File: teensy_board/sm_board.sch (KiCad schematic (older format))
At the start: 45 parts, among them J0 CONN_01X03, J1 CONN_01X03, J10 CONN_01X04, J11 CONN_01X02, J12 CONN_02X04, J2 CONN_01X03, J3 CONN_01X03, J4 CONN_01X03, J5 CONN_01X03, J6 CONN_01X03, J7 CONN_01X02, J8 CONN_01X02, J9 CONN_01X04, U1 Teensy3.6, U2 drv8833, U3 tps82130

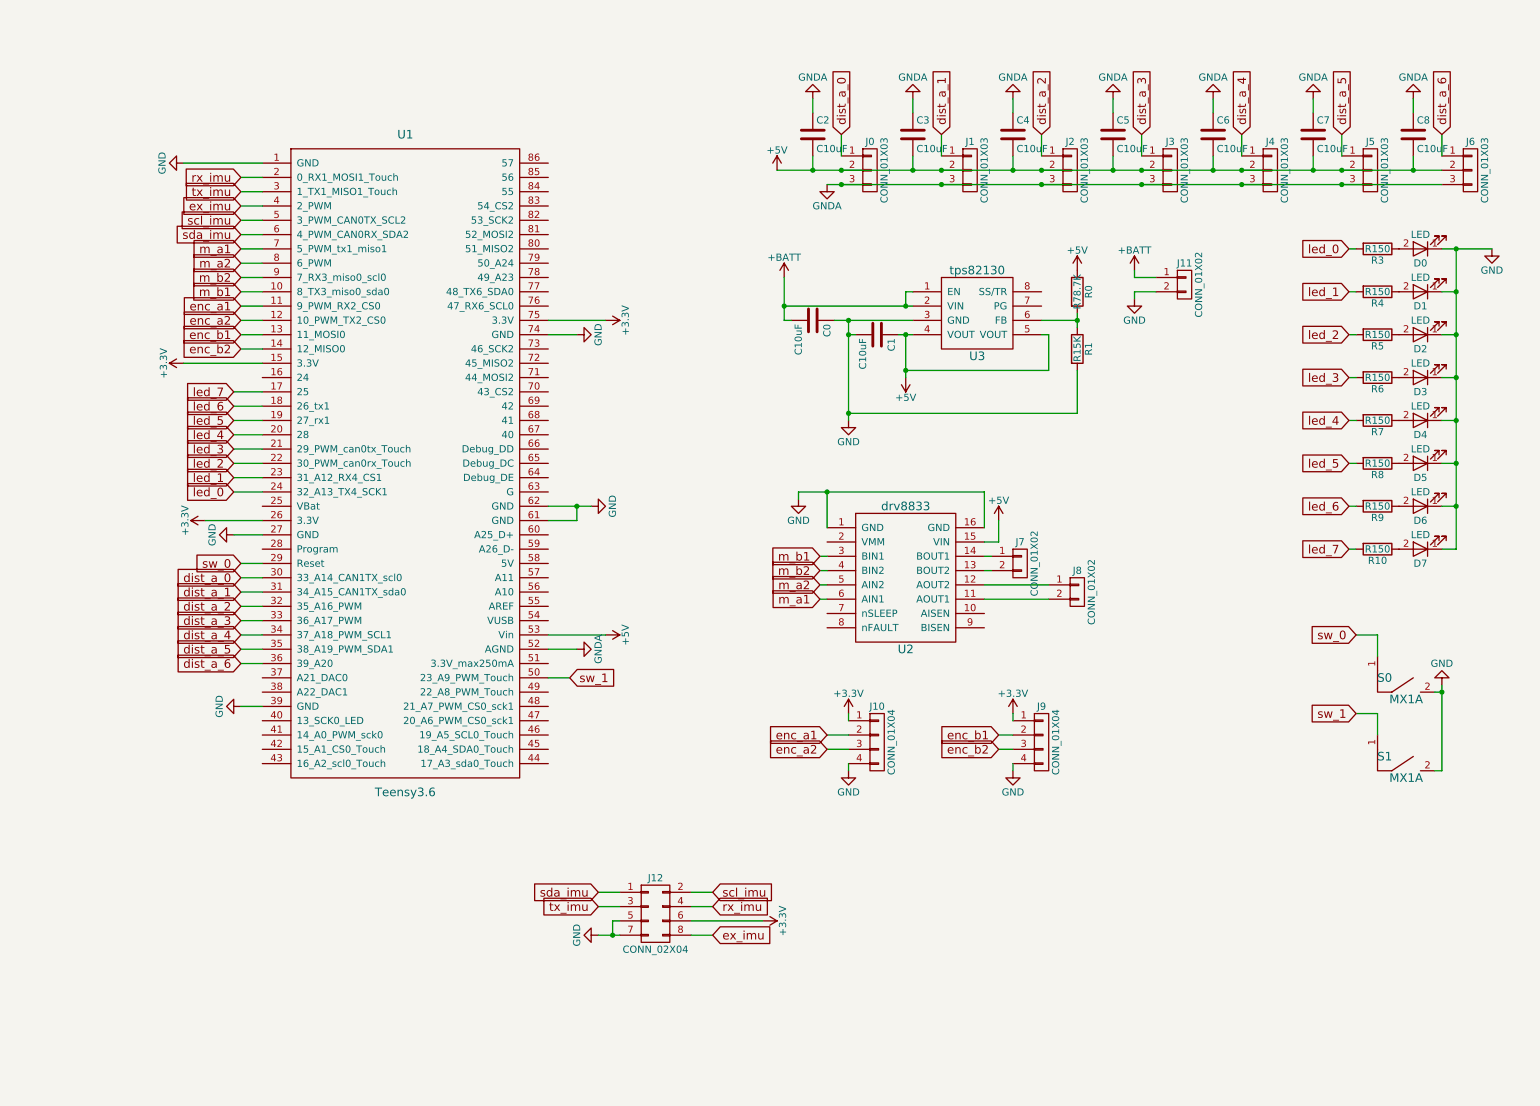
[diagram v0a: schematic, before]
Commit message: I think im done the schematic for tonight
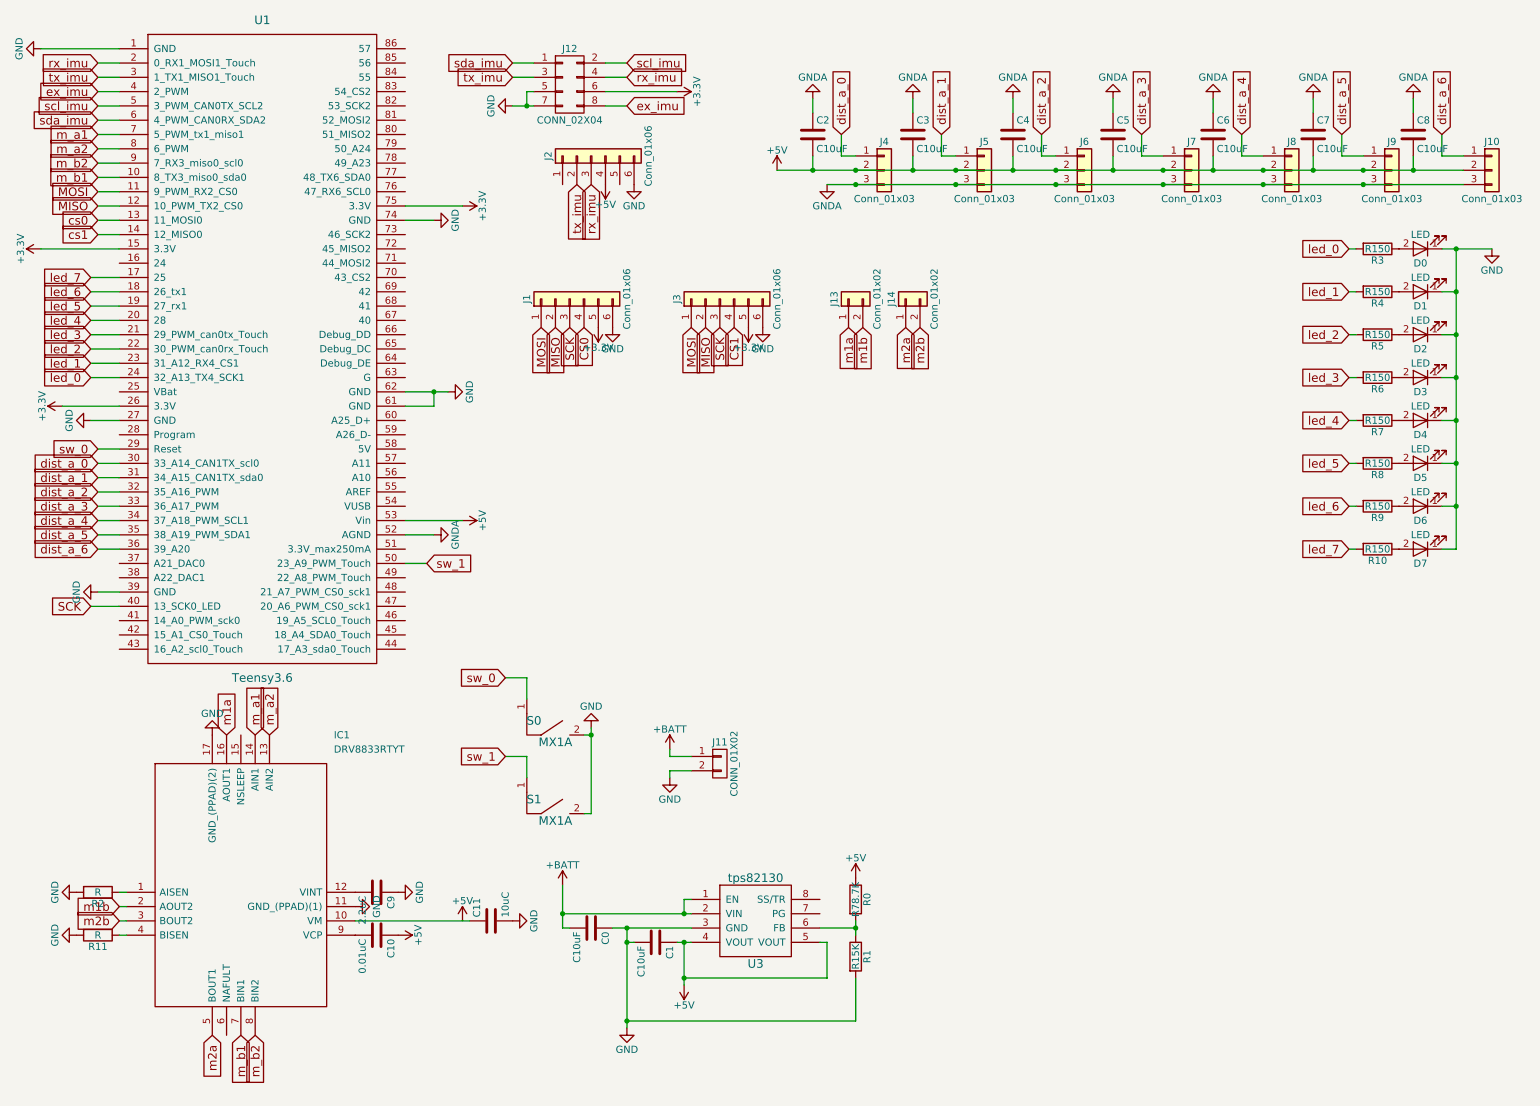
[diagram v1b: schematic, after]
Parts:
- removed J0, J1, J2, J3, J4, J5, J6: CONN_01X03, Pin_Headers:Pin_Header_Straight_1x03_Pitch2.54mm, symbol CONN_01X03
- removed J10, J9: CONN_01X04, Pin_Headers:Pin_Header_Straight_1x04_Pitch2.54mm, symbol CONN_01X04
- removed J7, J8: CONN_01X02, Pin_Headers:Pin_Header_Straight_1x02_Pitch2.54mm, symbol CONN_01X02
- removed U2: drv8833, drv8833:drv8833, symbol drv8833
- added C10: 0.01uC, Capacitors_SMD:C_0603, symbol C
- added C11: 10uC, Capacitors_SMD:C_0603, symbol C
- added C9: 2.2uC, Capacitors_SMD:C_0603, symbol C
- added IC1: DRV8833RTYT, Housings_DFN_QFN:WQFN-16-1EP_4x4mm_Pitch0.65mm, symbol DRV8833RTYT
- added J1, J3: Conn_01x06, Connector_Molex:Molex_CLIK-Mate_502386-0670_1x06_P1.25mm_Horizontal, symbol Conn_01x06
- added J10, J4, J5, J6, J7, J8, J9: Conn_01x03, Connector_Molex:Molex_CLIK-Mate_502386-0370_1x03_P1.25mm_Horizontal, symbol Conn_01x03
- added J13, J14: Conn_01x02, Connector_Molex:Molex_CLIK-Mate_502494-0270_1x02_P2.00mm_Horizontal, symbol Conn_01x02
- added J2: Conn_01x06, Pin_Headers:Pin_Header_Straight_1x06_Pitch2.54mm, symbol Conn_01x06
- added R11, R2: R, Resistors_SMD:R_0603, symbol R
- C0, C1, C2, C3, C4, C5, C6, C7, C8: footprint Capacitors_SMD:C_0805 -> Capacitors_SMD:C_0603
- D0, D1, D2, D3, D4, D5, D6, D7: footprint LEDs:LED_0805 -> LEDs:LED_0603
- R0, R1, R10, R3, R4, R5, R6, R7, R8, R9: footprint Resistors_SMD:R_0805 -> Resistors_SMD:R_0603
- U1: footprint Teensy:Teensy35_36_custom -> Teensy:Teensy35_36
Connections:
- net +3V3: now also J1.5 (Pin_5), J3.5 (Pin_5)
- net +5V: now also C10.1, J10.2 (Pin_2), J2.4 (Pin_4), J4.2 (Pin_2), J5.2 (Pin_2), J6.2 (Pin_2), J7.2 (Pin_2), J8.2 (Pin_2), J9.2 (Pin_2)
- net GND: now also C11.2, C9.1, IC1.11 (GND_(PPAD)(1)), IC1.17 (GND_(PPAD)(2)), J1.6 (Pin_6), J2.6 (Pin_6), J3.6 (Pin_6), R11.2, R2.2
- net GNDA: now also J10.3 (Pin_3), J4.3 (Pin_3), J5.3 (Pin_3), J6.3 (Pin_3), J7.3 (Pin_3), J8.3 (Pin_3), J9.3 (Pin_3)
- net dist_a_0: now also J4.1 (Pin_1)
- net dist_a_1: now also J5.1 (Pin_1)
- net dist_a_2: now also J6.1 (Pin_1)
- net dist_a_3: now also J7.1 (Pin_1)
- net dist_a_4: now also J8.1 (Pin_1)
- net dist_a_5: now also J9.1 (Pin_1)
- net dist_a_6: now also J10.1 (Pin_1)
- net m_a1: now also IC1.14 (AIN1)
- net m_a2: now also IC1.13 (AIN2)
- net m_b1: now also IC1.7 (BIN1)
- net m_b2: now also IC1.8 (BIN2)
- net rx_imu: now also J2.3 (Pin_3)
- net tx_imu: now also J2.2 (Pin_2)
- net SCK: now reaches U1.40 (13_SCK0_LED)
- net SCK: now also J1.3 (Pin_3), J3.3 (Pin_3)
- net enc_a1 renamed MOSI
- net MOSI: now also J1.1 (Pin_1), J3.1 (Pin_1)
- net enc_a2 renamed MISO
- net MISO: now also J1.2 (Pin_2), J3.2 (Pin_2)
- net enc_b1 renamed cs0
- net enc_b2 renamed cs1
- new net: IC1.1 (AISEN), R2.1
- new net: C11.1, IC1.10 (VM)
- new net: C9.2, IC1.12 (VINT)
- new net: IC1.4 (BISEN), R11.1
- new net: C10.2, IC1.9 (VCP)
- new net CS0: J1.4 (Pin_4)
- new net CS1: J3.4 (Pin_4)
- new net m1a: IC1.16 (AOUT1), J13.1 (Pin_1)
- new net m1b: IC1.2 (AOUT2), J13.2 (Pin_2)
- new net m2a: IC1.5 (BOUT1), J14.1 (Pin_1)
- new net m2b: IC1.3 (BOUT2), J14.2 (Pin_2)
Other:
- moved on the sheet: C0, C1, J11, J12, R0, R1, S0, S1, U3
